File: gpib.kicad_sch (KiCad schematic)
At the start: 4 parts, among them U1 SN74LVC8T245PWR, U2 SN74LVC07APWR, U6 SN74LVC1G07DCKR, U7 SN74LVC14APWR

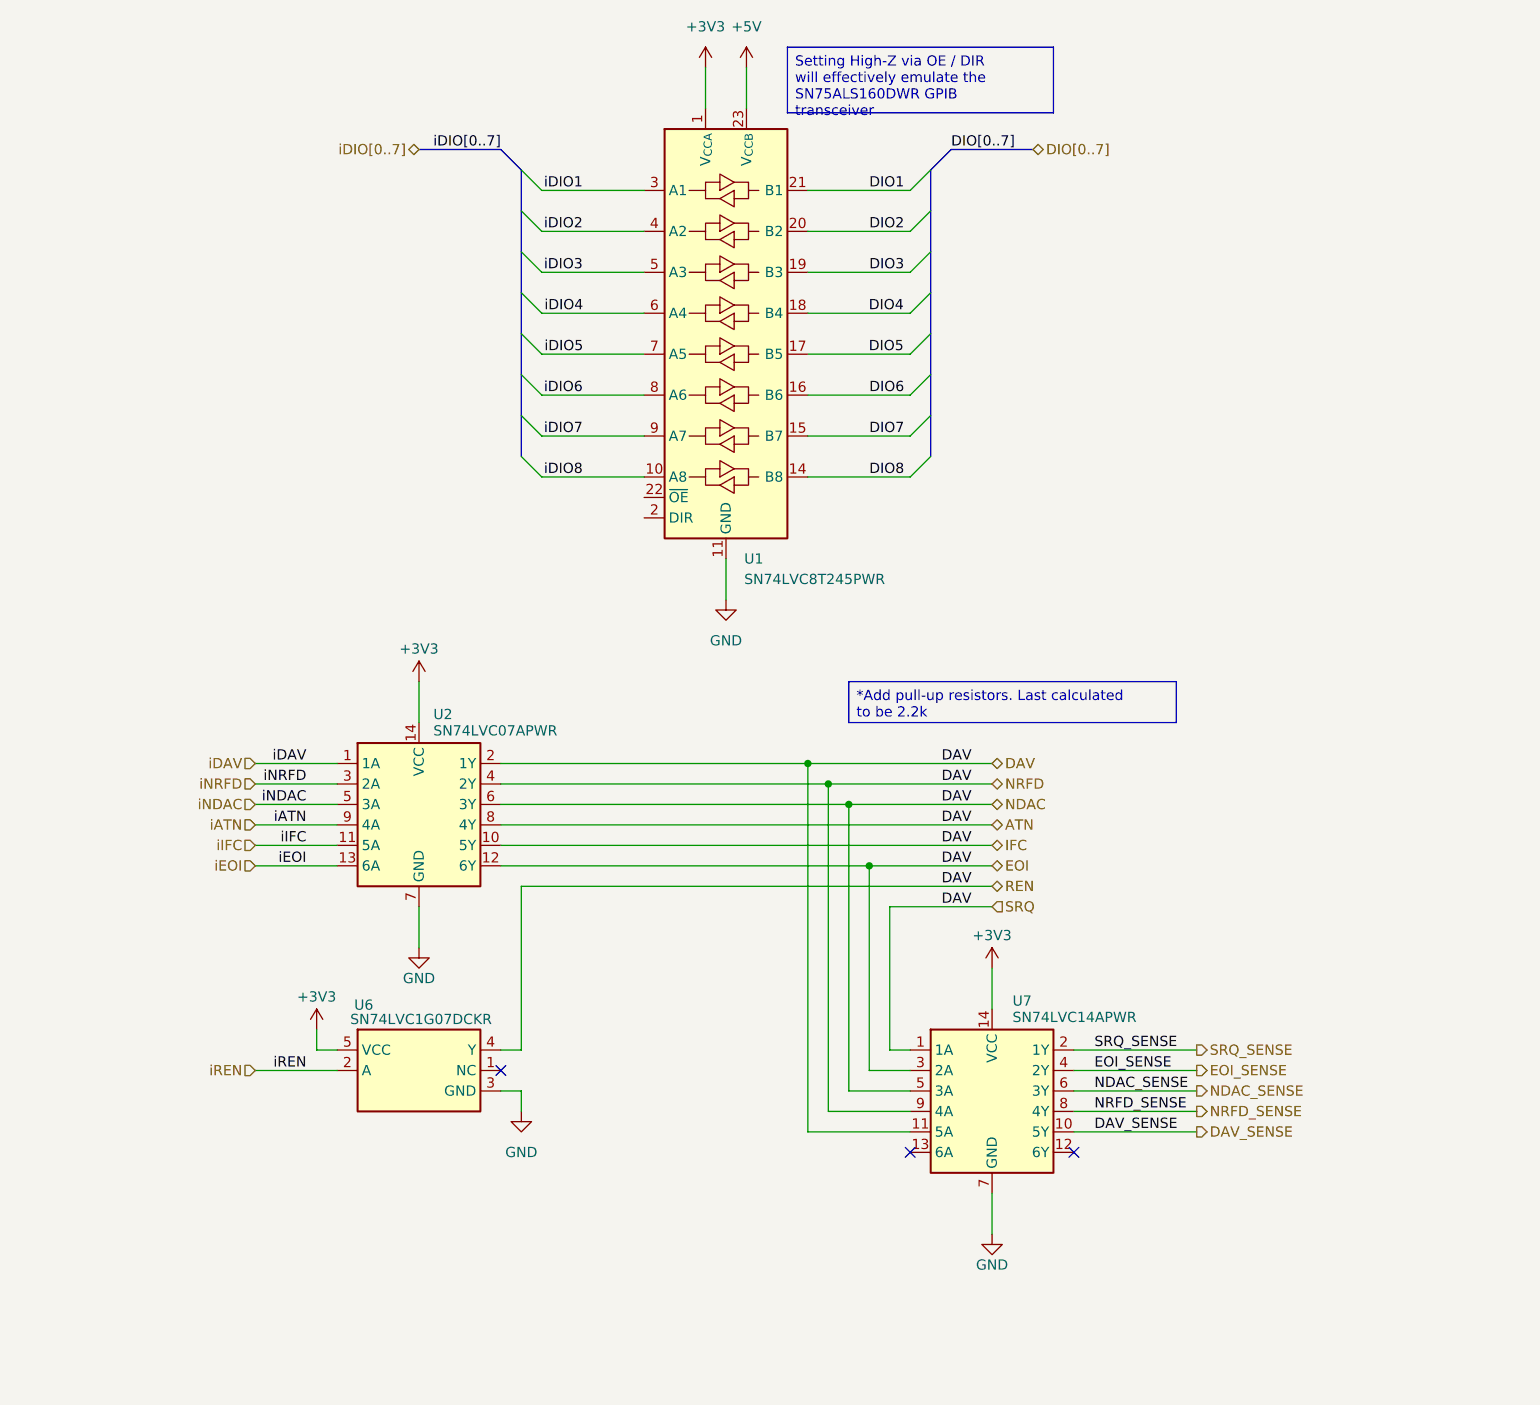
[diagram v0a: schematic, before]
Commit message: Finish up schematics
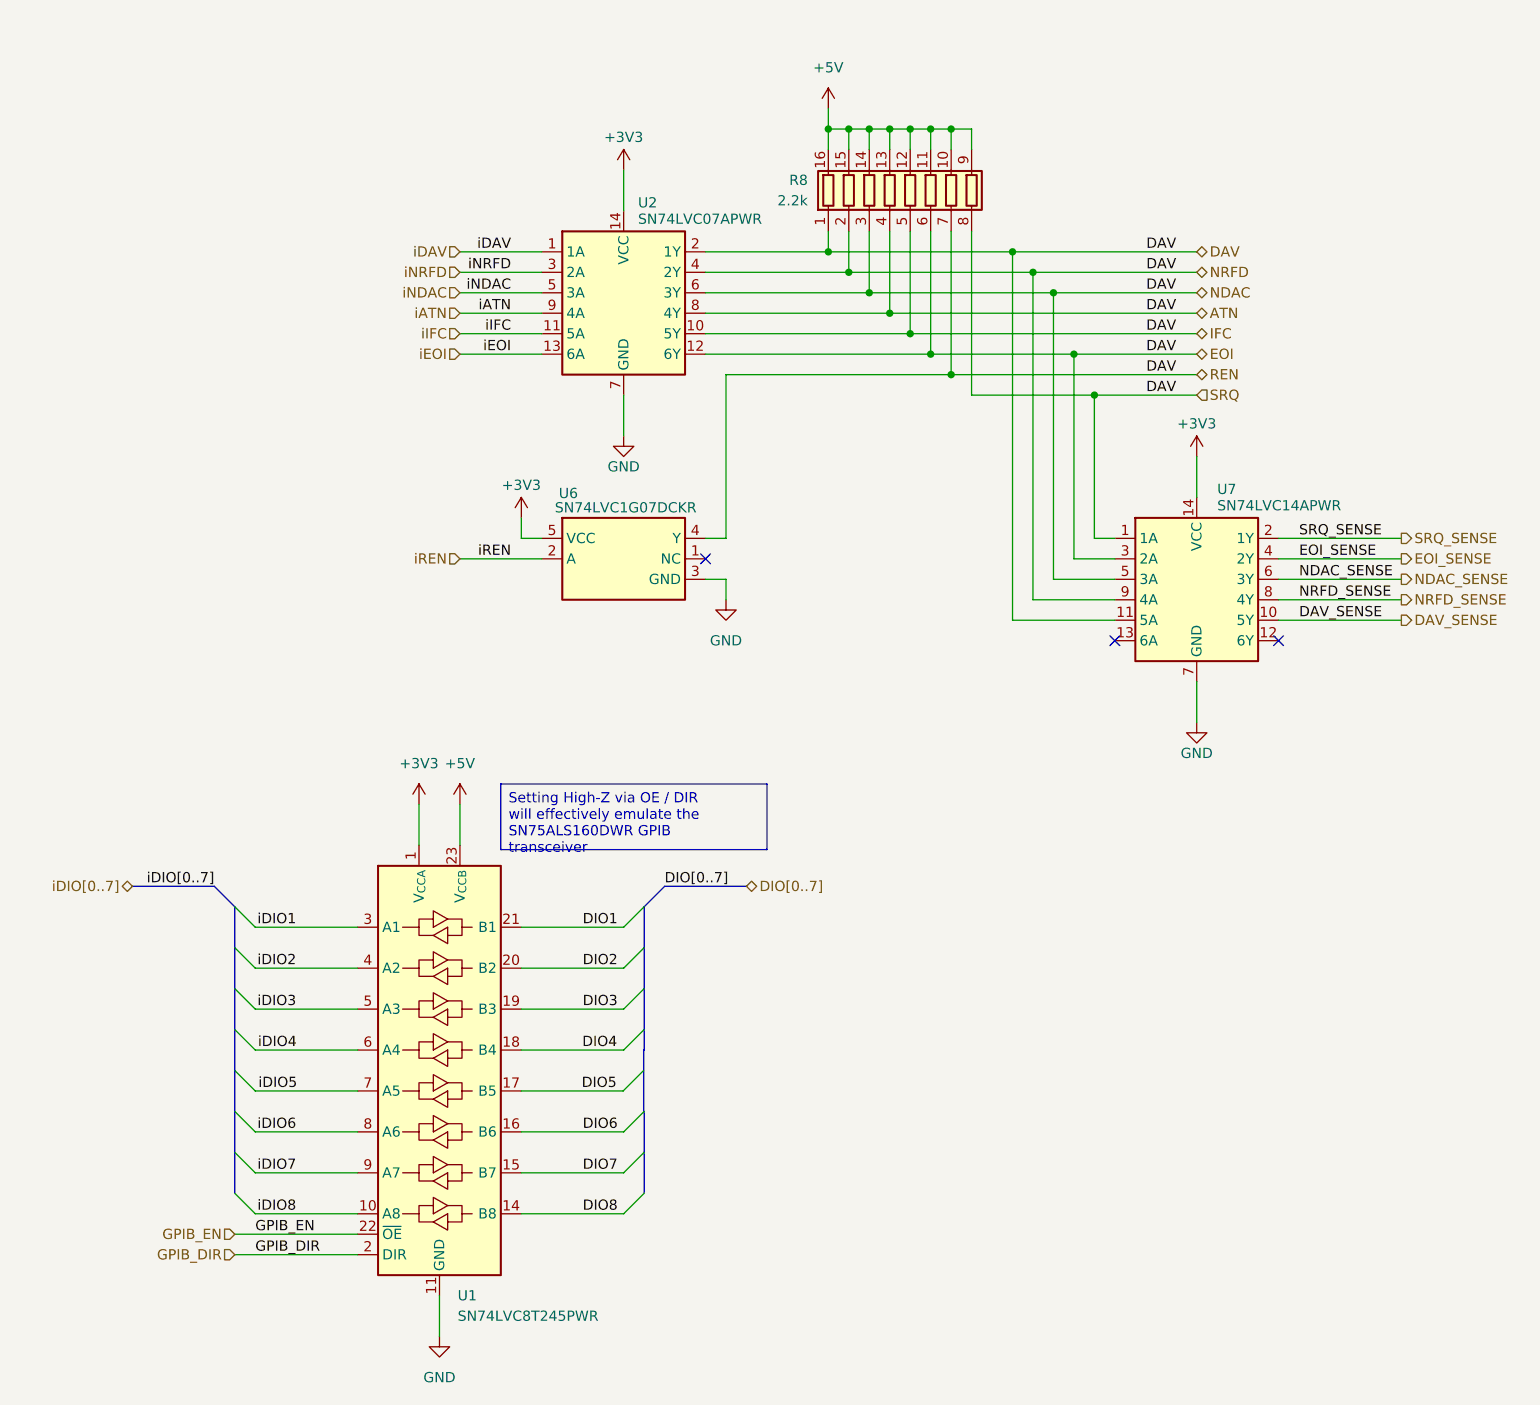
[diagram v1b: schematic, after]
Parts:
- added R8: 2.2k, Resistor_SMD:R_Array_Convex_8x0602, symbol PARTSDB:EXB-2HV222JV
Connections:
- net +5V: now also R8.10 (R7.2), R8.11 (R6.2), R8.12 (R5.2), R8.13 (R4.2), R8.14 (R3.2), R8.15 (R2.2), R8.16 (R1.2), R8.9 (R8.2)
- net ATN: now also R8.1 (R1.1), R8.2 (R2.1), R8.3 (R3.1), R8.4 (R4.1), R8.5 (R5.1), R8.6 (R6.1), R8.7 (R7.1), R8.8 (R8.1)
- net DIO5: now also U1.17 (B5)
- net iDIO5: now also U1.7 (A5)
- net GPIB_DIR: now reaches U1.2 (DIR)
- net GPIB_EN: now reaches U1.22 (~{OE})
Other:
- title: (none) -> GPIB Transceiver
- moved on the sheet: U1, U2, U6, U7
